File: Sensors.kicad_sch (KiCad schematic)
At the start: 23 parts, among them J2 Conn_Coaxial, U1 NEO-M8N

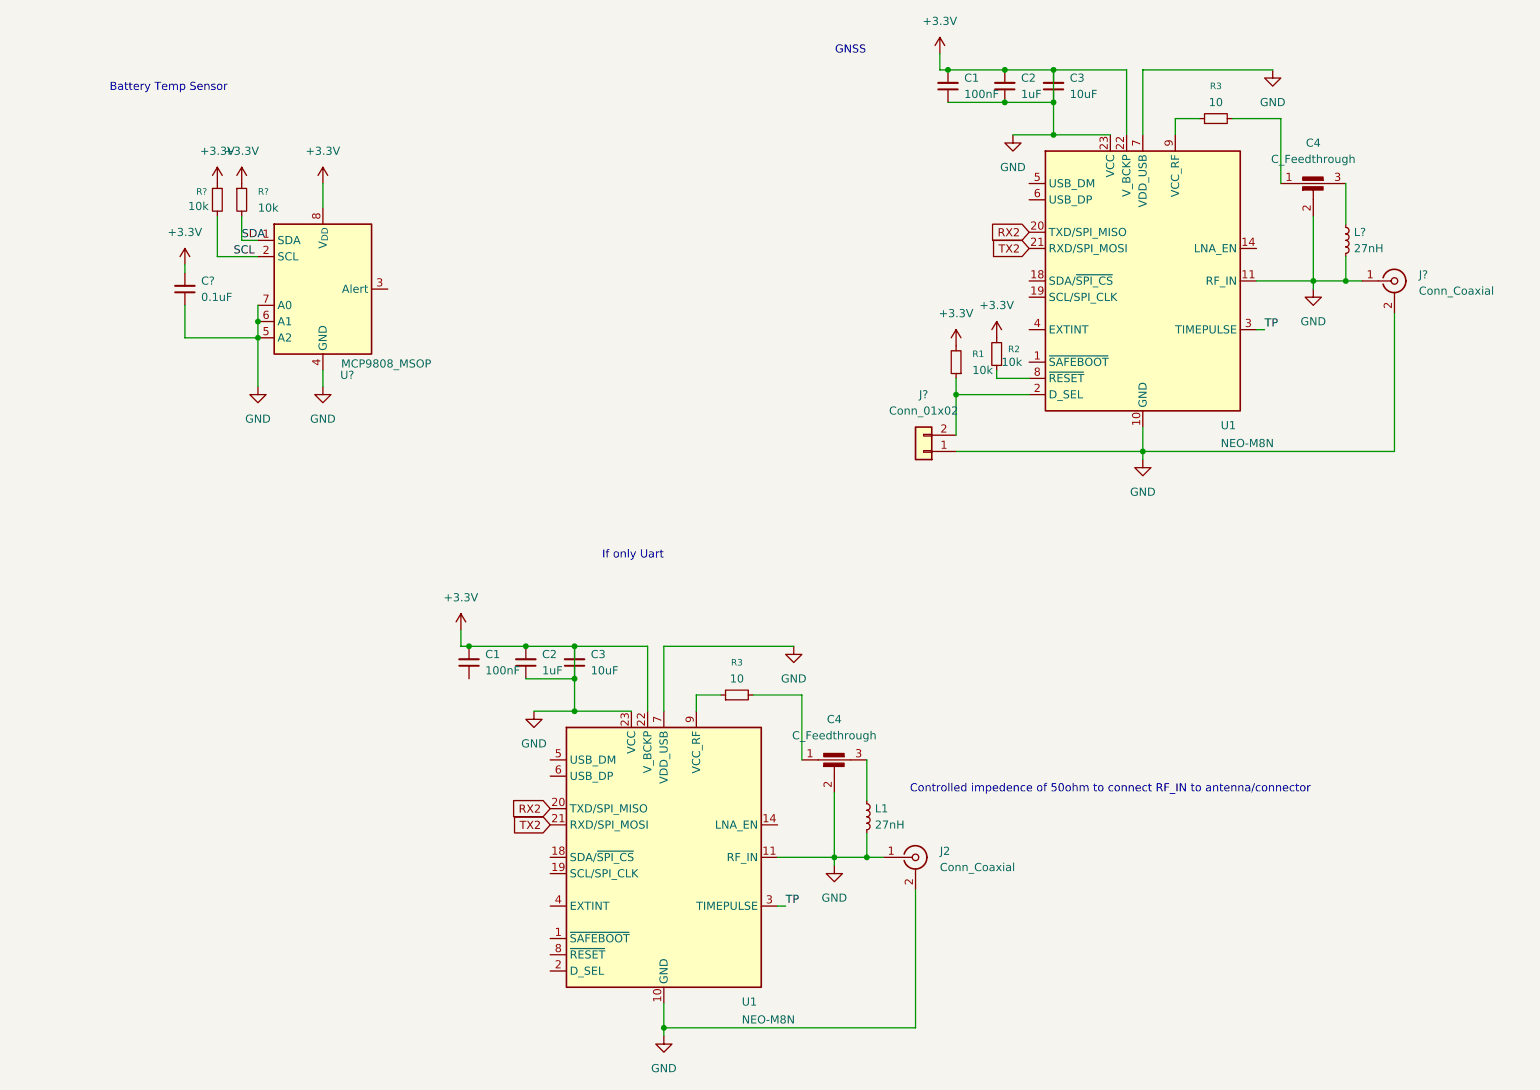
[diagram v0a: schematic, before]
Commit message: Sensors
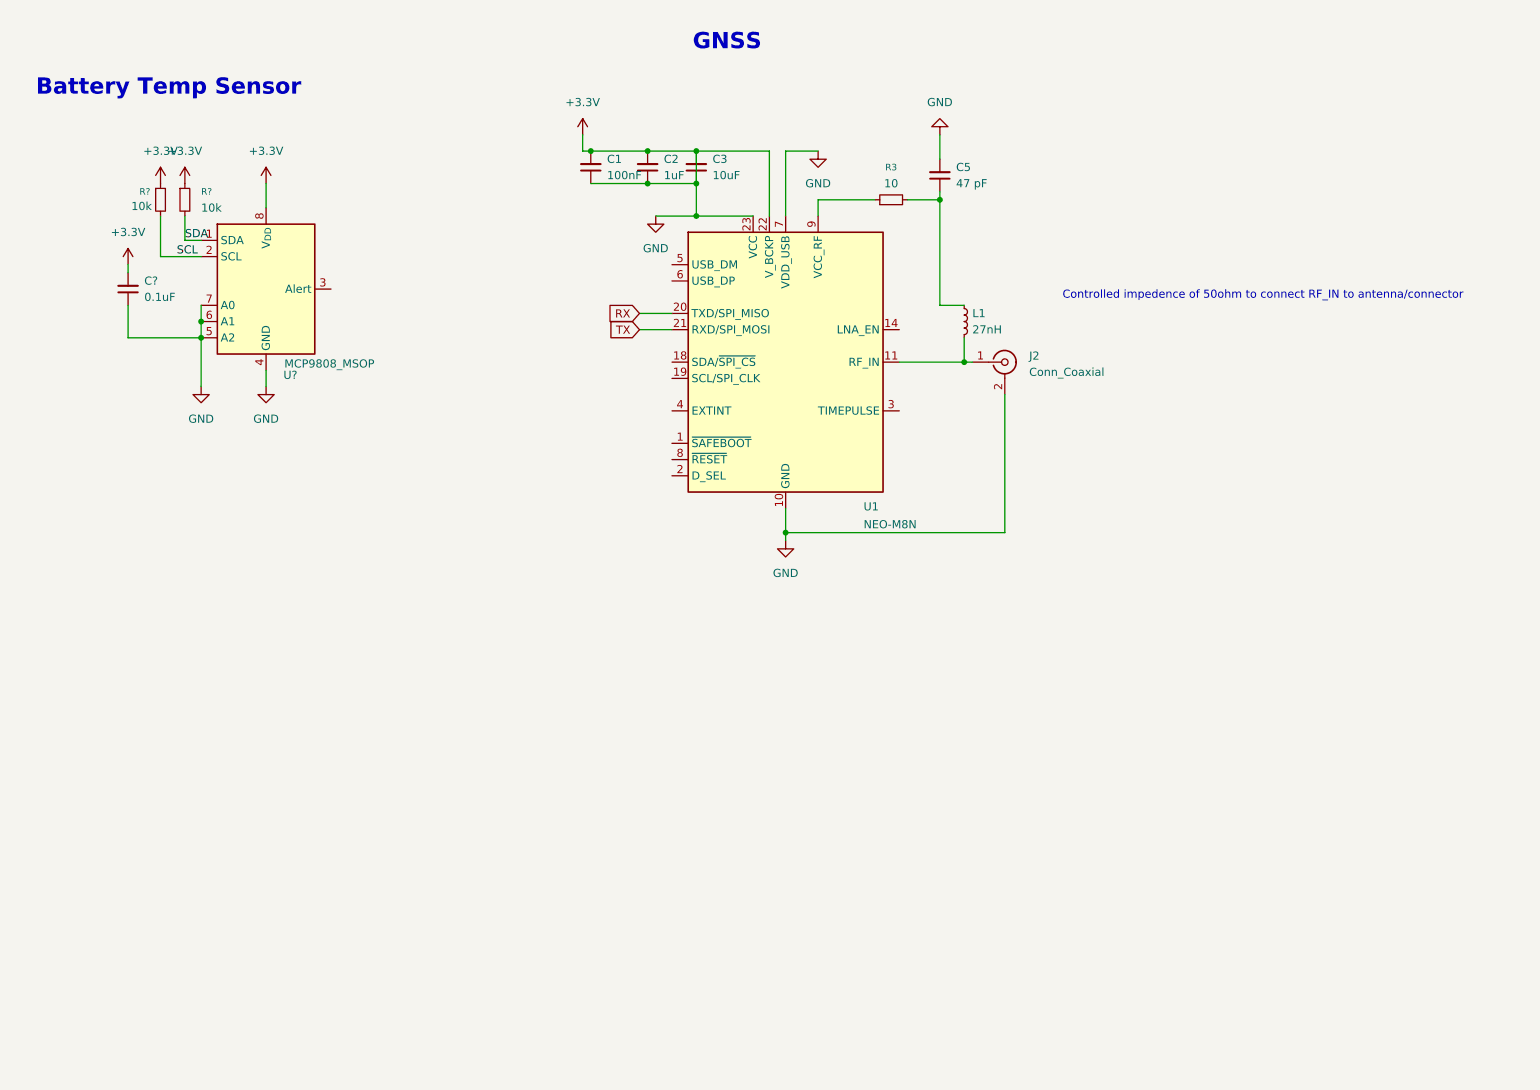
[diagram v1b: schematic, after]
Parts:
- removed C1: 100nF, symbol Device:C_Small
- removed C2: 1uF, symbol Device:C_Small
- removed C3: 10uF, symbol Device:C_Small
- removed C4 (x2): C_Feedthrough, symbol Device:C_Feedthrough
- removed J?: Conn_01x02, Connector_JST:JST_XH_B1B-XH-AM_1x01_P2.50mm_Vertical, symbol Connector_Generic:Conn_01x02
- removed J?: Conn_Coaxial, symbol Connector:Conn_Coaxial
- removed L?: 27nH, symbol Device:L_Small
- removed R1, R2: 10k, symbol Device:R_Small
- removed R3: 10, symbol Device:R_Small
- removed U1: NEO-M8N, RF_GPS:ublox_NEO, symbol RF_GPS:NEO-M8N
- added C5: 47 pF, symbol Device:C_Small
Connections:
- net +3.3V: now also C1.1, C5.2; no longer J2.1 (In), L1.2, U1.11 (RF_IN)
- net at R3.2: now also L1.1, C5.1
- net RX2 renamed RX
- net TP: no longer names the net of U1.3 (TIMEPULSE)
- net TX2 renamed TX
- new net: J2.1 (In), L1.2, U1.11 (RF_IN)
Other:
- note removed: "If only Uart"
- moved on the sheet: C1, C2, C3, C?, J2, L1, R3, R?, U1, U?
